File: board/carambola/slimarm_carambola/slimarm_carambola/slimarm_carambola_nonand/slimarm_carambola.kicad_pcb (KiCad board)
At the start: 4 copper layers, 49.2 x 28 mm, 72 parts, among them J1 USB_C_Receptacle_USB2.0, J2 Conn_01x04, J4 DF13A-7P-1.25H21, SW1 SW_MEC_5E, U1 AT91SAM9G25-CU, U2 16bit-DDR2-8bank-FBGA84, U3 W25Q128JVS, U5 XC6206PxxxMR, U6 XC6206PxxxMR, U7 XC6206PxxxMR, U8 XC6206PxxxMR, Y1 Crystal

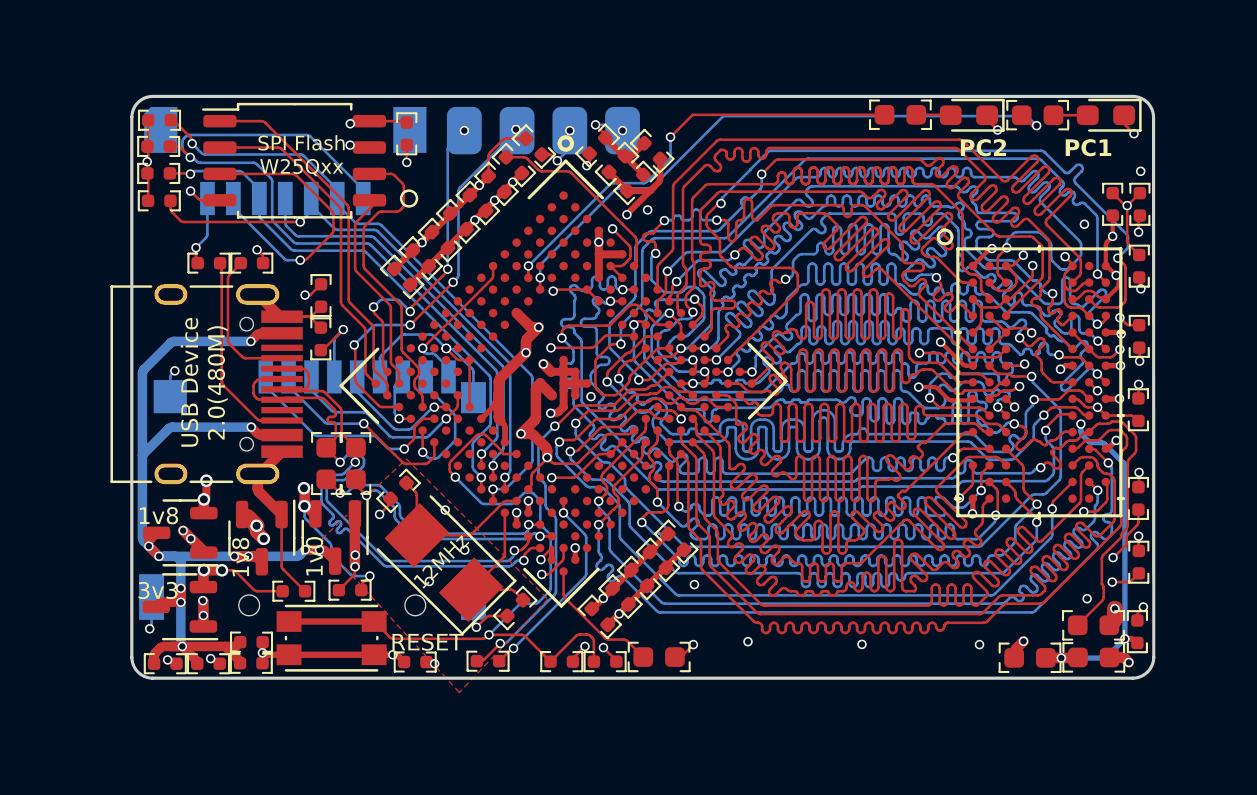
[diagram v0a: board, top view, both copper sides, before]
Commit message: 23x20f
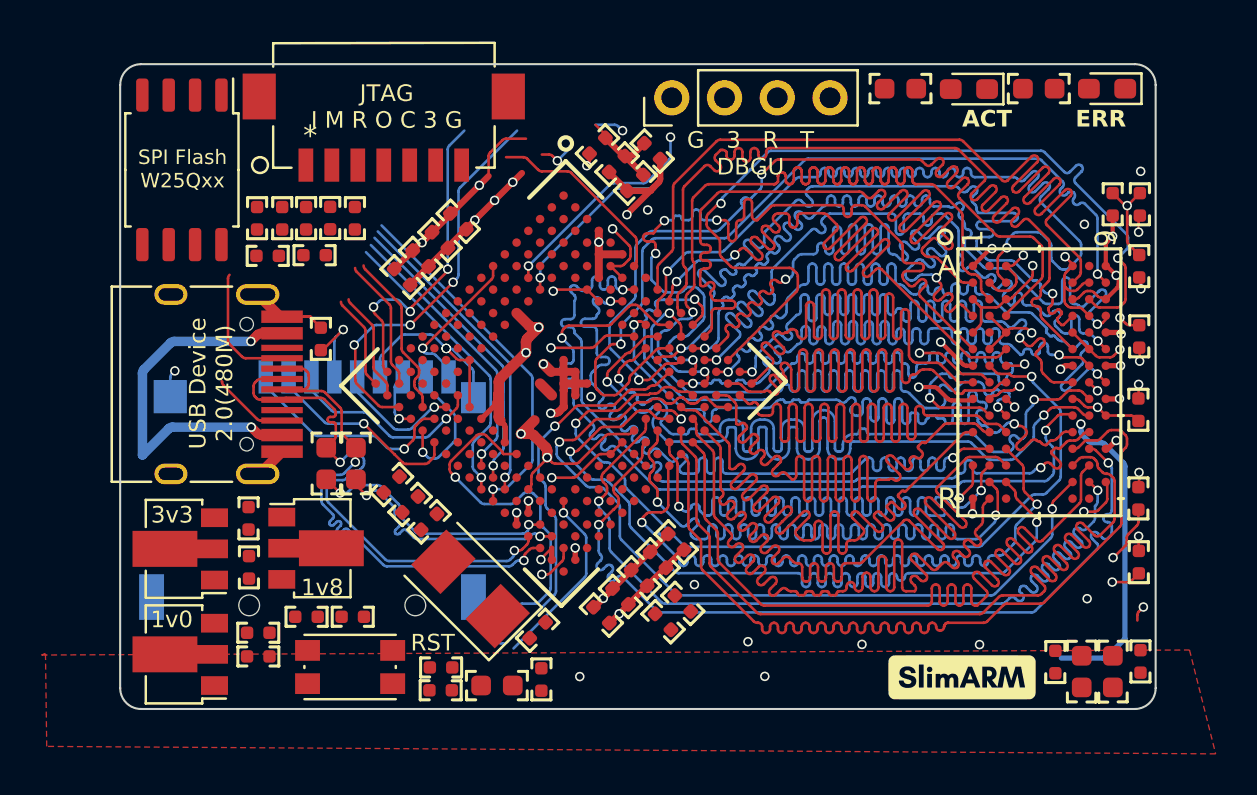
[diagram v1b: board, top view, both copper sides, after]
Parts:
- removed C35, C36: 22pF, jlywxy:0402
- removed the G*** at (27.6, 20.6)
- removed R12: 470k, jlywxy:0603
- removed U6: XC6206PxxxMR, Package_TO_SOT_SMD:SOT-23-3
- added C17: 22pF, jlywxy:0402, F.Cu at (60.3, 40.7)
- added G***: LOGO, LOGO, F.Cu at (55.8, 41.4)
- added G***: LOGO, jlywxy:image_slimarm, B.Cu at (56.1, 32.0)
- added G***: LOGO, jlywxy:image_monazite_baremetal, B.Cu at (35.8, 32.7)
- J2, J4: moved to F.Cu
- U5: value XC6206PxxxMR -> AMS1117; footprint Package_TO_SOT_SMD:SOT-23-3 -> Package_TO_SOT_SMD:SOT-89-3
- U7, U8: footprint Package_TO_SOT_SMD:SOT-23-3 -> Package_TO_SOT_SMD:SOT-89-3
- moved G*** 33.7 mm to (52.8, 28.3)
- moved G*** 32.3 mm to (59.8, 27.0)
- moved C5 22.1 mm to (42.3, 37.9)
- moved C4 22.0 mm to (41.4, 38.8)
- moved C6 17.7 mm to (28.3, 32.2), turned to 45 degrees
- moved R9 17.1 mm to (29.2, 33.1), turned to 45 degrees
- moved R24 9.69 mm to (26.5, 19.3), turned to -90 degrees
- moved U8 9.59 mm to (17.8, 40.3), turned to 180 degrees
- moved R22 8.49 mm to (24.2, 19.3), turned to -90 degrees
- moved C27 8.28 mm to (21.8, 19.3), turned to -90 degrees
- moved R23 8.27 mm to (25.4, 19.3), turned to -90 degrees
- moved C33 8.07 mm to (21.4, 33.8), turned to 90 degrees
- moved R3 7.93 mm to (33.4, 41.8), turned to 0 degrees
- moved R11 7.90 mm to (30.7, 41.0)
- moved R13 6.88 mm to (23.0, 19.3), turned to -90 degrees
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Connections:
- C10 pad 2: /1v8_CPUMEM -> /1v8_DDR
- C11 pad 2: /1v8_CPUMEM -> /1v8_DDR
- C9 pad 2: /1v8_CPUMEM -> /1v8_DDR
- R10 pad 2: /1v8_CPUMEM -> /3v3
- U1 pad D10: /1v8_CPUMEM -> /1v8_DDR
- U1 pad D13: /1v8_CPUMEM -> /1v8_DDR
- U1 pad F14: /1v8_CPUMEM -> /1v8_DDR
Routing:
- net /1v8_CPUMEM: track 85.7 -> 0.00 mm, vias 8 -> 0
- net /1v8_DDR: track 137.5 -> 216.5 mm, vias 24 -> 23
- net GND: track 135.5 -> 96.4 mm, vias 63 -> 39
- net +5V: track 51.4 -> 18.9 mm, vias 11 -> 2
- net /3v3: track 106.9 -> 77.2 mm, vias 20 -> 12
- net /JTAG_TDI: track 37.4 -> 13.4 mm, vias 2 -> 1
- net Net-(U1A-PC1): track 29.1 -> 8.11 mm, vias 2 -> 1
- net Net-(SW1-A): track 35.6 -> 18.3 mm, vias 2 -> 1
- net /DDR_CS: track 54.5 -> 41.6 mm
- net /JTAG_TMS: track 30.1 -> 17.4 mm, vias 2 -> 1
- net /JTAG_RST: track 27.4 -> 15.1 mm, vias 2 -> 1
- net /SPI_CS: track 17.3 -> 5.34 mm
- net /JTAG_TCK: track 26.2 -> 14.4 mm, vias 2 -> 1
- net /SPI_MISO: track 15.7 -> 4.59 mm
- net Net-(U1A-PC2): track 21.3 -> 10.5 mm
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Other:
- board size 49.2 x 28 mm -> 49.9 x 31.1 mm
- board text added: "ACT ERR"
- board text added: "Carambola v1r1x259 AT91SAM9G25@400MHz github: jlywxy/slimarm"
- board text added: "Classic"
- board text added: "RST"
- board text removed: "12MHz"
- board text removed: "Carambola v1r0x202 AT91SAM9G25@400MHz github: jlywxy/slimarm"
- board text removed: "Micro SD DET: PC8"
- board text removed: "PC2 PC1"
- board text removed: "RESET"
- board text removed: "SlimARM Classic"
